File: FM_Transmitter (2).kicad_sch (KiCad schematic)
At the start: 18 parts, among them J1 AudioJack2_Ground, U1 MAX2606

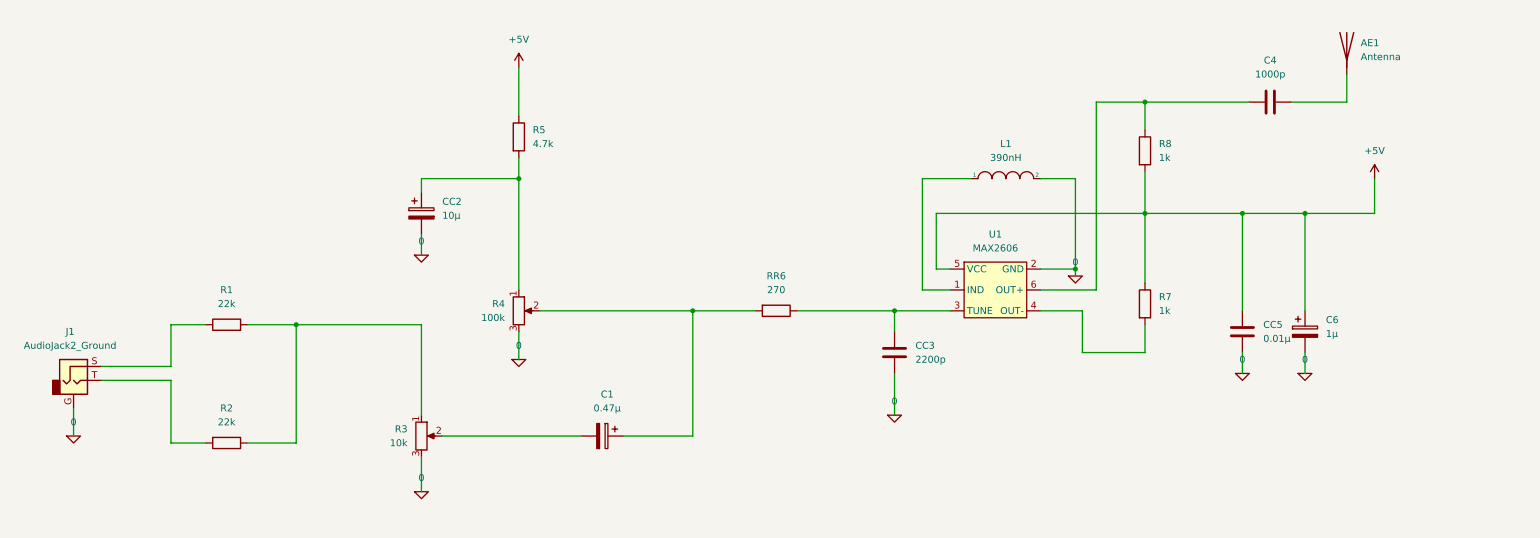
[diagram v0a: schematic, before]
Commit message: kontrolle Board bitte
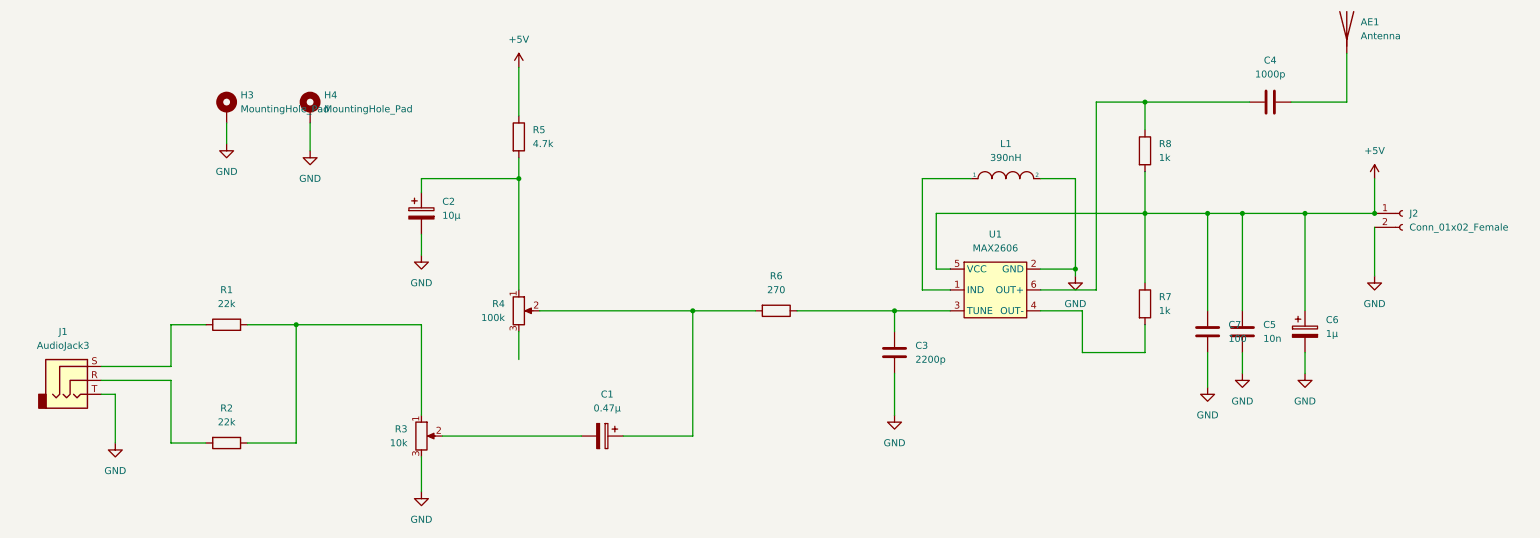
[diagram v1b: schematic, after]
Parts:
- removed J1: AudioJack2_Ground, symbol Connector:AudioJack2_Ground
- added C7: 100, Capacitor_SMD:C_0805_2012Metric, symbol Device:C
- added H3, H4: MountingHole_Pad, MountingHole:MountingHole_2.2mm_M2_DIN965_Pad, symbol Mechanical:MountingHole_Pad
- added J1: AudioJack3, Connector_Audio:Jack_3.5mm_CUI_SJ-3523-SMT_Horizontal, symbol Connector:AudioJack3
- added J2: Conn_01x02_Female, Connector_PinSocket_2.00mm:PinSocket_1x02_P2.00mm_Vertical, symbol Connector:Conn_01x02_Female
- AE1: footprint (none) -> Connector_Wire:SolderWire-0.1sqmm_1x01_D0.4mm_OD1mm_Relief
- C1, C6: footprint (none) -> Capacitor_SMD:CP_Elec_3x5.3
- C2: renamed from CC2; footprint (none) -> Capacitor_SMD:CP_Elec_3x5.3
- C3: renamed from CC3; footprint (none) -> Capacitor_SMD:C_0805_2012Metric
- C4: footprint (none) -> Capacitor_SMD:C_0805_2012Metric
- C5: renamed from CC5; value 0.01µ -> 10n; footprint (none) -> Capacitor_SMD:CP_Elec_3x5.3
- L1: footprint (none) -> Inductor_SMD:L_0805_2012Metric
- R1, R2: footprint Resistor_SMD:R_1206_3216Metric -> Resistor_SMD:R_0805_2012Metric
- R3, R4: footprint (none) -> Potentiometer_SMD:Potentiometer_ACP_CA6-VSMD_Vertical
- R5, R7, R8: footprint (none) -> Resistor_SMD:R_0805_2012Metric
- R6: renamed from RR6; footprint (none) -> Resistor_SMD:R_0805_2012Metric
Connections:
- net +5V: now also C7.1, J2.1 (Pin_1)
- net at R1.1: now also J1.S
- net at R2.2: now also J1.R
- net 0 renamed GND
- net GND: now also C7.2, H3.1, H4.1, J1.T, J2.2 (Pin_2); no longer R4.3
